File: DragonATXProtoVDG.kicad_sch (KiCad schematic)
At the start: 64 parts, among them IC1 74LS273, J1 Conn_Coaxial, J3 JTAG, U1 AD724JR, U3 ATF1508AS-10JI84, Y2 4.433618MHz, Y3 100MHz

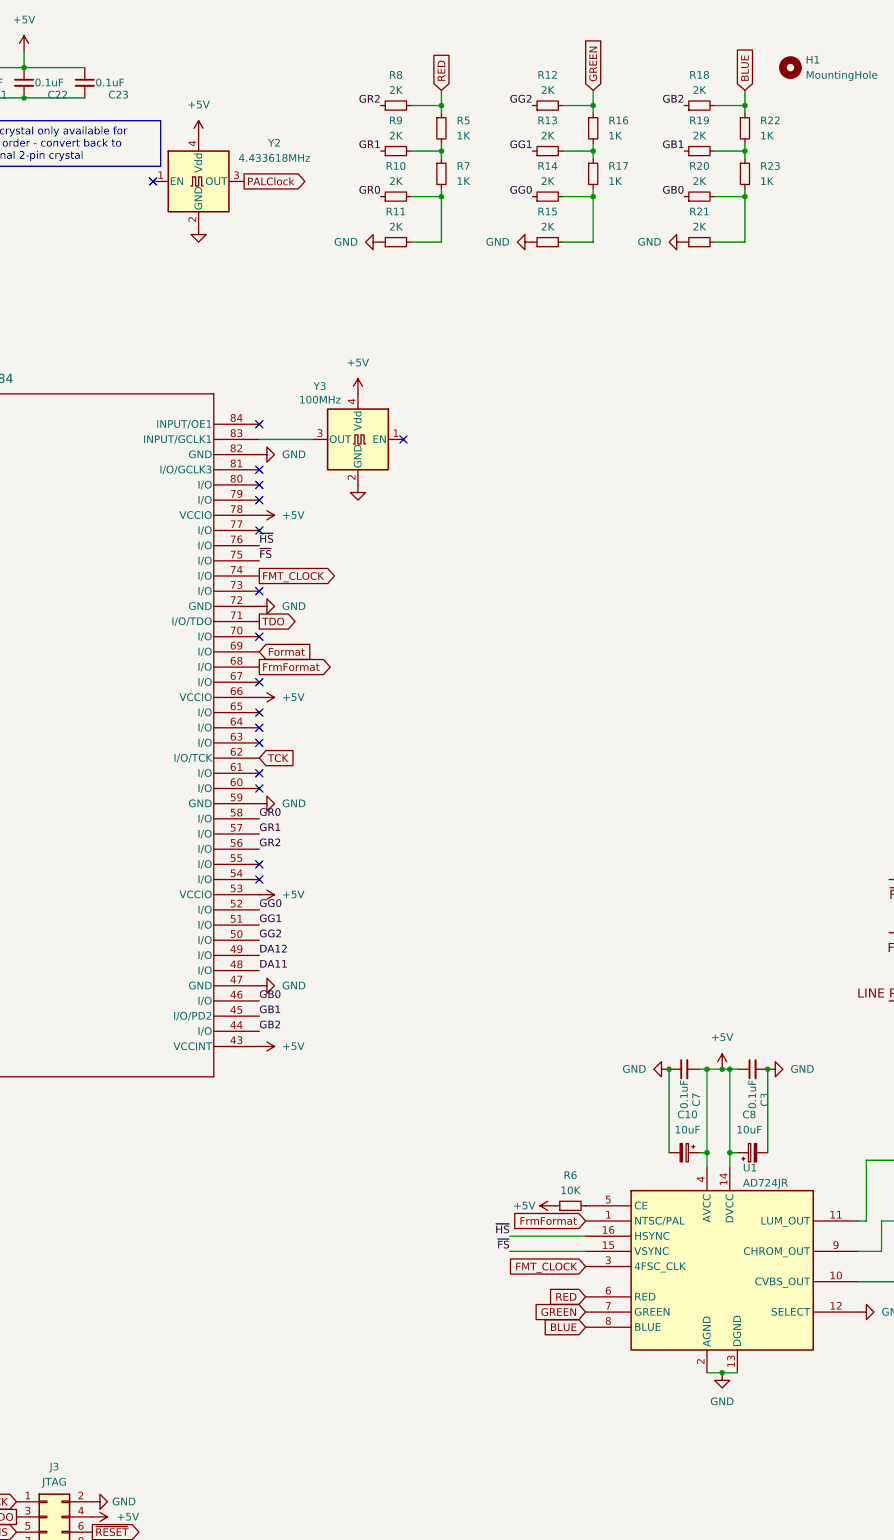
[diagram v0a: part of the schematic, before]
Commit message: revise for 1.0.7
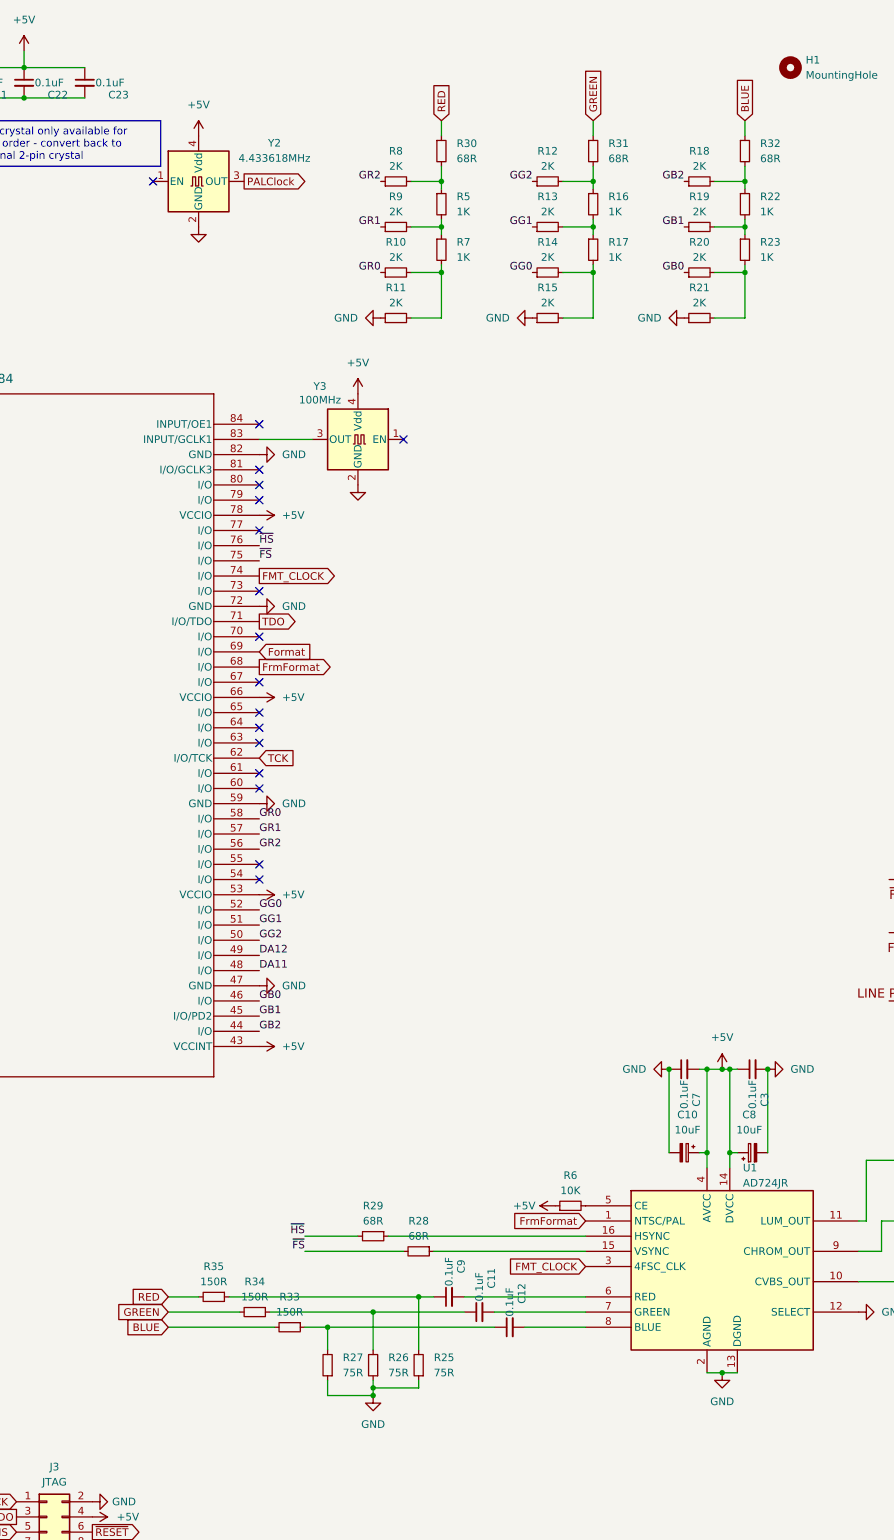
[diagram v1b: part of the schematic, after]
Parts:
- added C11, C12, C9: 0.1uF, Capacitor_SMD:C_0805_2012Metric_Pad1.18x1.45mm_HandSolder, symbol Device:C_Small
- added R25, R26, R27: 75R, PCM_Resistor_SMD_AKL:R_0805_2012Metric_Pad1.15x1.40mm_HandSolder, symbol Device:R_Small
- added R28, R29, R30, R31, R32: 68R, PCM_Resistor_SMD_AKL:R_0805_2012Metric_Pad1.15x1.40mm_HandSolder, symbol Device:R_Small
- added R33, R34, R35: 150R, PCM_Resistor_SMD_AKL:R_0805_2012Metric_Pad1.15x1.40mm_HandSolder, symbol Device:R_Small
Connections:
- net BLUE: now also R32.1, R33.2; no longer R18.2, R22.1, U1.8 (BLUE)
- net GND: now also R25.1, R26.1, R27.1
- net GREEN: now also R31.1, R34.2; no longer R12.2, R16.1, U1.7 (GREEN)
- net RED: now also R30.1, R35.2; no longer R5.1, R8.2, U1.6 (RED)
- net ~{FS}: now also R28.2; no longer U1.15 (VSYNC)
- net ~{HS}: now also R29.2; no longer U1.16 (HSYNC)
- new net: R30.2, R5.1, R8.2
- new net: R18.2, R22.1, R32.2
- new net: R12.2, R16.1, R31.2
- new net: C9.1, R25.2, R35.1
- new net: C11.1, R26.2, R34.1
- new net: R28.1, U1.15 (VSYNC)
- new net: C11.2, U1.7 (GREEN)
- new net: R29.1, U1.16 (HSYNC)
- new net: C9.2, U1.6 (RED)
- new net: C12.2, U1.8 (BLUE)
- new net: C12.1, R27.2, R33.1
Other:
- moved on the sheet: R10, R11, R12, R13, R14, R15, R16, R17, R18, R19, R20, R21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
